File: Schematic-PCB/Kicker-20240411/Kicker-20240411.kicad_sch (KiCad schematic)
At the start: 23 parts, among them J1 Conn_01x02_Pin, J2 Conn_01x05_Pin, J3 Conn_01x02_Pin, Q1 NMOS, U2 TSSP58P38, U3 TSSP58P38, U4 74LVC1G04, U5 74LVC1G04, U6 74AHC1G08

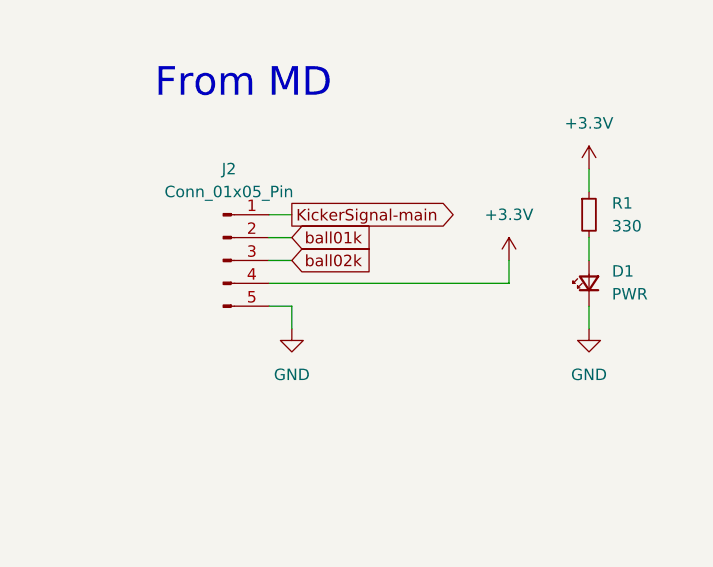
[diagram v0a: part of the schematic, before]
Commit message: Auto stash before merge of "main" and "origin/main"
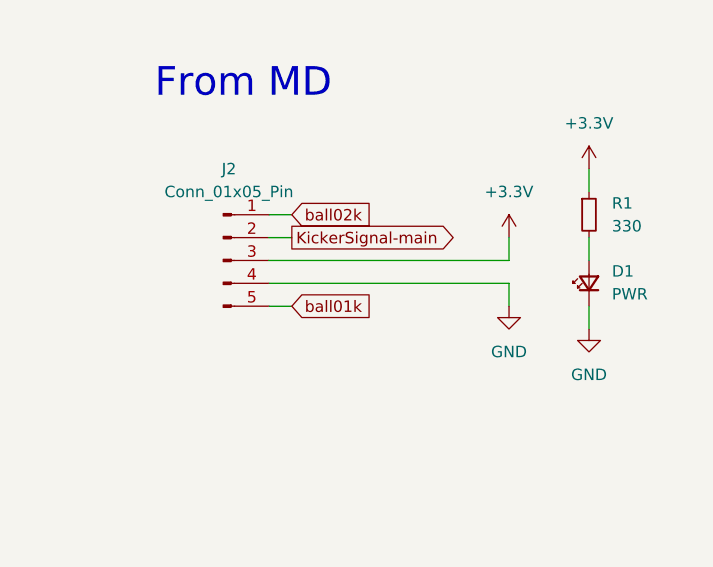
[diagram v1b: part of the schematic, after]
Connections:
- net +3.3V: now also J2.3 (Pin_3); no longer J2.4 (Pin_4)
- net GND: now also J2.4 (Pin_4); no longer J2.5 (Pin_5)
- net KickerSignal-main: now also J2.2 (Pin_2); no longer J2.1 (Pin_1)
- net ball01k: now also J2.5 (Pin_5); no longer J2.2 (Pin_2)
- net ball02k: now also J2.1 (Pin_1); no longer J2.3 (Pin_3)
